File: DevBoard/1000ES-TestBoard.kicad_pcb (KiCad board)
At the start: 2 copper layers, 57 parts, among them J10 KeyPad_IN, J11 D.AUDIO_OUT, J12 USB_C_CONTROL, J13 USB_C_AUDIO, J14 USB_C_DISPLAY, J4 from CNP401-B, J5 SONY Controls, J6 fromCNP401, J7 Power_IN, J8 Display_Out, J9 KeyPad_OUT, U10 TCA8418RTWR, U11 CONTROLLER_ESP, U12 AUDIO_ESP, U13 MCP1825S-3302E_AB, U14 DISLPAY_ESP, U6 SN74AHCT245, U7 SN74AHCT245, U8 SN74AHCT245, U9 SN74AHCT245

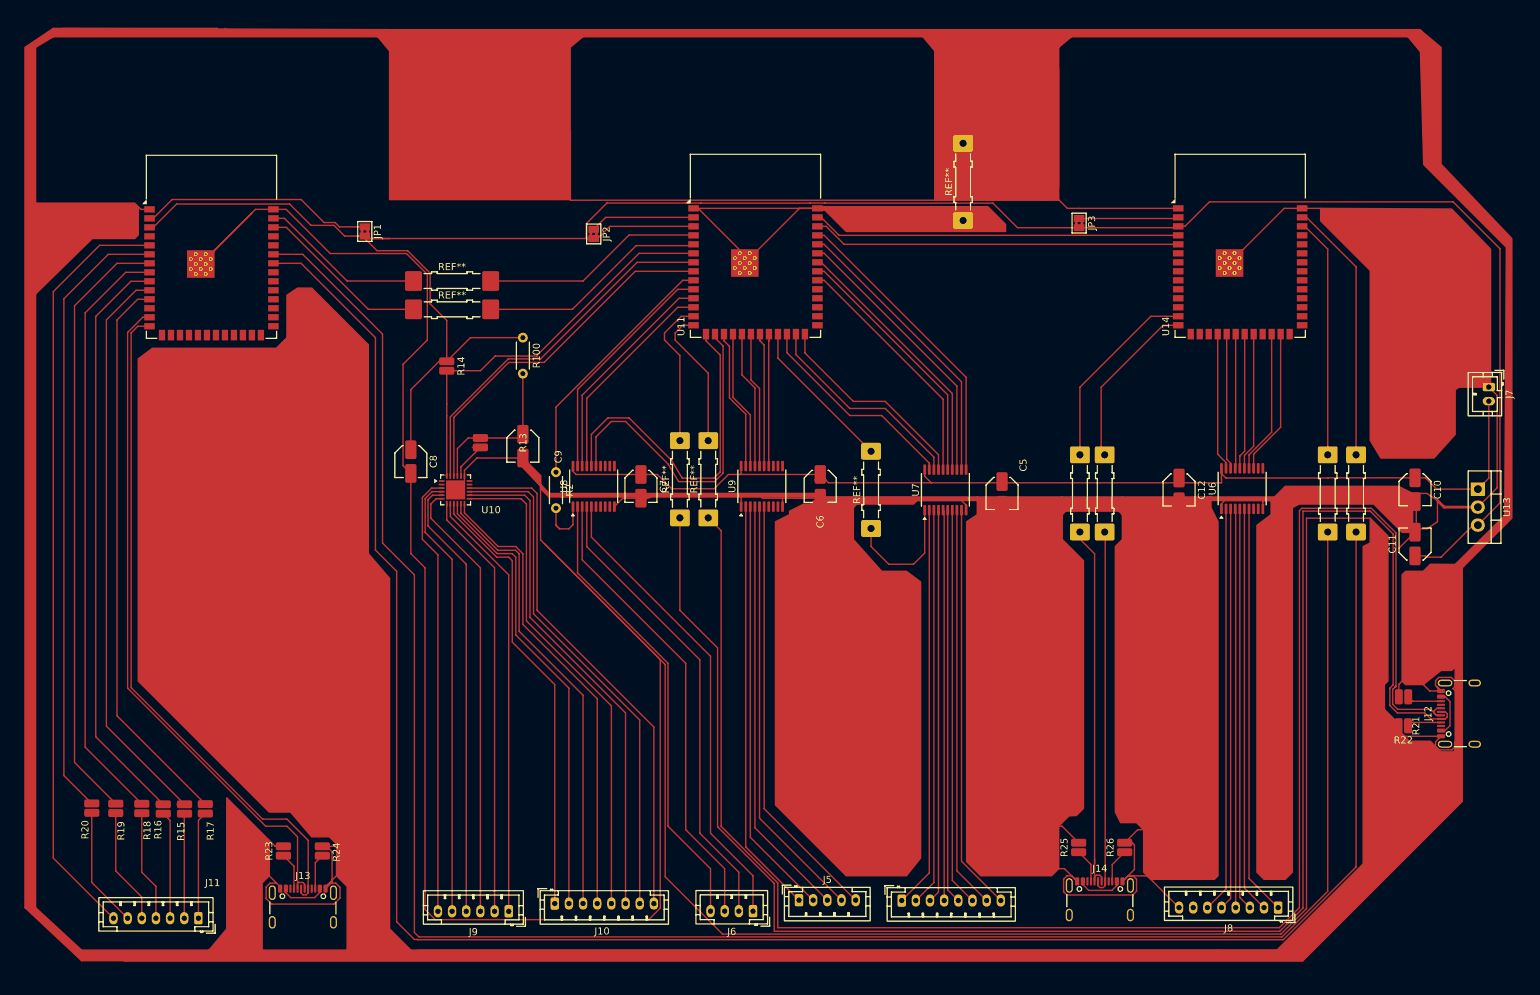
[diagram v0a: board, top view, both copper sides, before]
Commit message: Add files via upload
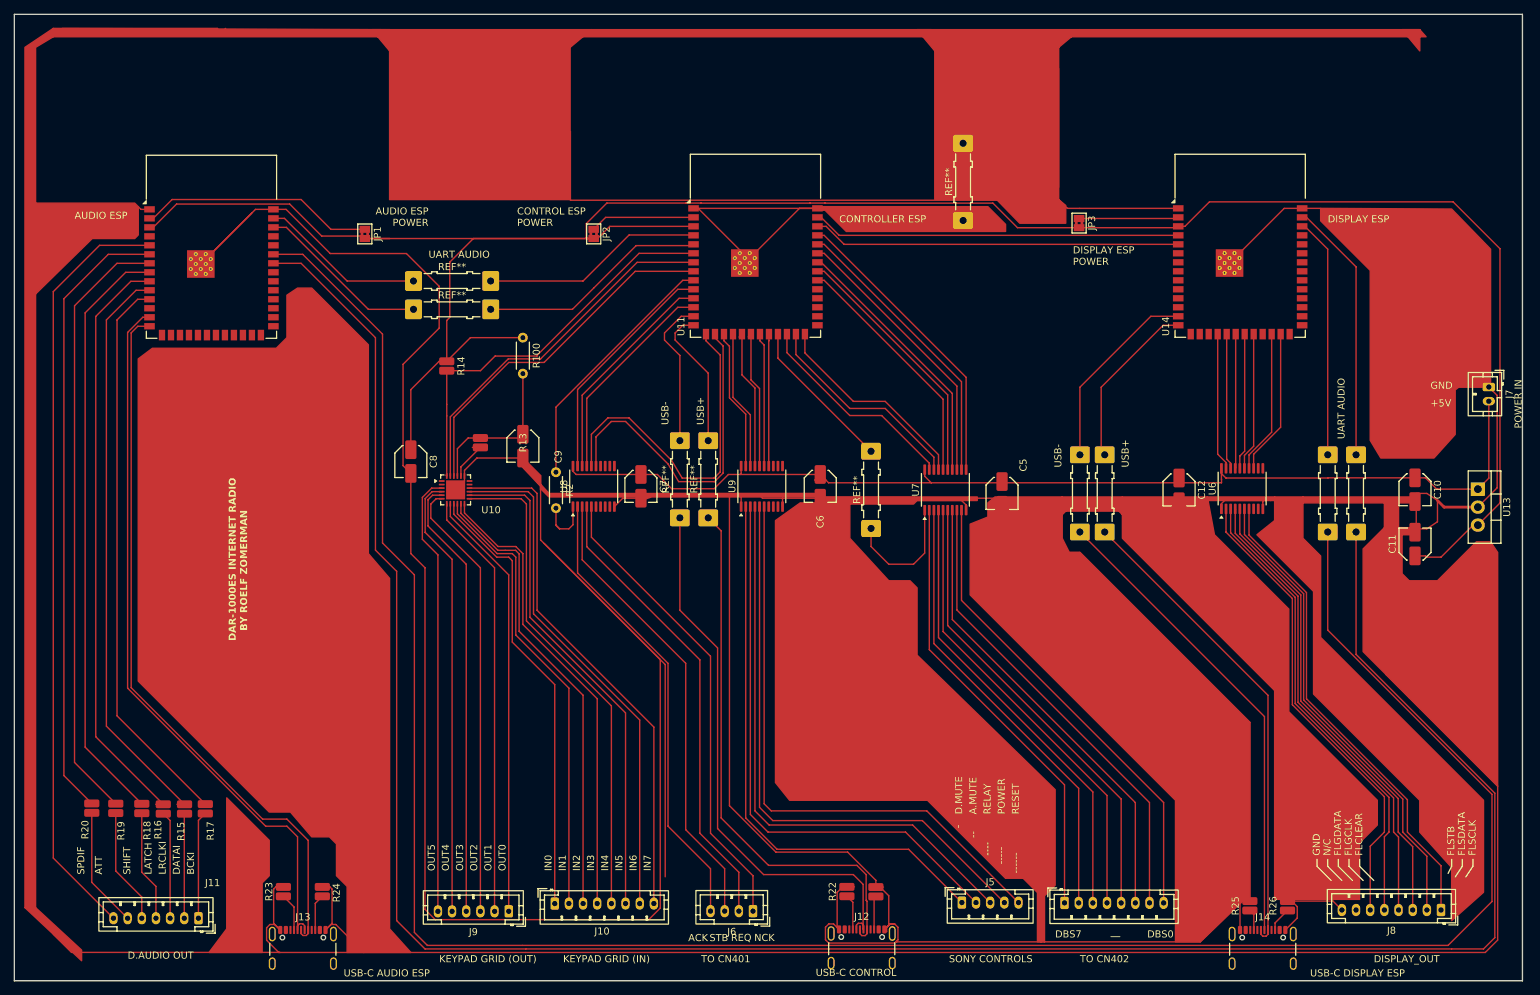
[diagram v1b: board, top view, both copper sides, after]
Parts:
- J5: value SONY Controls -> fromVariousPoints
- REF**: value UDB- -> USB-
- moved J12 92.1 mm to (157.7, 150.4), turned to 0 degrees
- moved R22 82.0 mm to (155.6, 141.4), turned to 90 degrees
- moved R21 79.4 mm to (159.7, 141.4), turned to 90 degrees
- moved R25 25.5 mm to (212.5, 143.4)
- moved R26 24.4 mm to (217.8, 143.4)
- moved J14 24.0 mm to (214.3, 150.5)
- moved J4 23.0 mm to (186.3, 143.0)
- moved J5 23.0 mm to (171.8, 142.9)
- moved J8 23.0 mm to (239.5, 144.0)
- moved J13 5.84 mm to (78.8, 150.5)
- moved R23 5.74 mm to (76.0, 141.4)
- moved R24 5.74 mm to (81.5, 141.4)
- moved JP1 0.35 mm to (87.5, 48.5)
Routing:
- net /ES1000-Default/USB_D-_prog1: track 266.1 -> 99.9 mm
- net /ES1000-Default/USB_D+_prog1: track 262.9 -> 97.4 mm
- net GND: track 1079.1 -> 1213.5 mm
- net /ES1000-Default/TXD_prog2: track 327.7 -> 231.5 mm
- net /ES1000-Default/RXD_prog2: track 323.1 -> 227.0 mm
- net /ES1000-Default/RESET: track 60.9 -> 83.7 mm
- net /ES1000-Default/POWER: track 60.4 -> 82.6 mm
- net /ES1000-Default/RELAY: track 59.8 -> 81.6 mm
- net /ES1000-Default/A.MUTE: track 59.3 -> 80.5 mm
- net /ES1000-Default/D.MUTE: track 58.7 -> 79.4 mm
- net +5V: track 173.7 -> 155.3 mm
- net /ES1000-Default/USB_D+_prog3: track 76.1 -> 93.1 mm
- net /ES1000-Default/USB_D-_prog3: track 81.7 -> 95.0 mm
- net +3.3V: track 309.9 -> 320.3 mm
- net /ES1000-Default/FLCLEAR: track 56.3 -> 66.3 mm
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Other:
- board outline added: 213 x 136.5 mm
- board text added: "+5V"
- board text added: "-"
- board text added: "--"
- board text added: "----"
- board text added: "-----"
- board text added: "------"
- board text added: "A.MUTE"
- board text added: "ACK"
- board text added: "ATT"
- board text added: "AUDIO ESP"
- board text added: "AUDIO ESP POWER"
- board text added: "BCKI"
- board text added: "CONTROL ESP POWER"
- board text added: "CONTROLLER ESP"
- board text added: "D.AUDIO OUT"
- board text added: "D.MUTE"
- board text added: "DAR-1000ES INTERNET RADIO BY ROELF ZOMERMAN"
- board text added: "DATAI"
- board text added: "DBS0"
- board text added: "DBS7"
- board text added: "DISPLAY ESP"
- board text added: "DISPLAY ESP POWER"
- board text added: "DISPLAY_OUT"
- board text added: "FLCLEAR"
- board text added: "FLGCLK"
- board text added: "FLGDATA"
- board text added: "FLSCLK"
- board text added: "FLSDATA"
- board text added: "FLSTB"
- board text added: "GND"
- board text added: "IN0"
- board text added: "IN1"
- board text added: "IN2"
- board text added: "IN3"
- board text added: "IN4"
- board text added: "IN5"
- board text added: "IN6"
- board text added: "IN7"
- board text added: "KEYPAD GRID (IN)"
- board text added: "KEYPAD GRID (OUT)"
- board text added: "LATCH"
- board text added: "LRCLKI"
- board text added: "N/C"
- board text added: "NCK"
- board text added: "OUT0"
- board text added: "OUT1"
- board text added: "OUT2"
- board text added: "OUT3"
- board text added: "OUT4"
- board text added: "OUT5"
- board text added: "POWER"
- board text added: "POWER IN"
- board text added: "RELAY"
- board text added: "REQ"
- board text added: "RESET"
- board text added: "SHIFT"
- board text added: "SONY CONTROLS"
- board text added: "SPDIF"
- board text added: "STB"
- board text added: "TO CN401"
- board text added: "TO CN402"
- board text added: "UART AUDIO"
- board text added: "USB+"
- board text added: "USB-"
- board text added: "USB-C AUDIO ESP"
- board text added: "USB-C CONTROL"
- board text added: "USB-C DISPLAY ESP"
- board text added: "|"
